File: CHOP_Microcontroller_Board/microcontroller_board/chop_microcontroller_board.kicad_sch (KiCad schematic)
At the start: 33 parts, among them J11 HEATER_SIGNAL_1, J12 POWER_HEAT, J14 BatteryToMainBoard, J2 OLED, J3 Encoder, J6 PFLOW, J7 DISC PUMP, J8 RTC, U1 Teensy4.1_Mounted, U2 U3V50F24, U3 U3V50F12, U4 D36V6F5

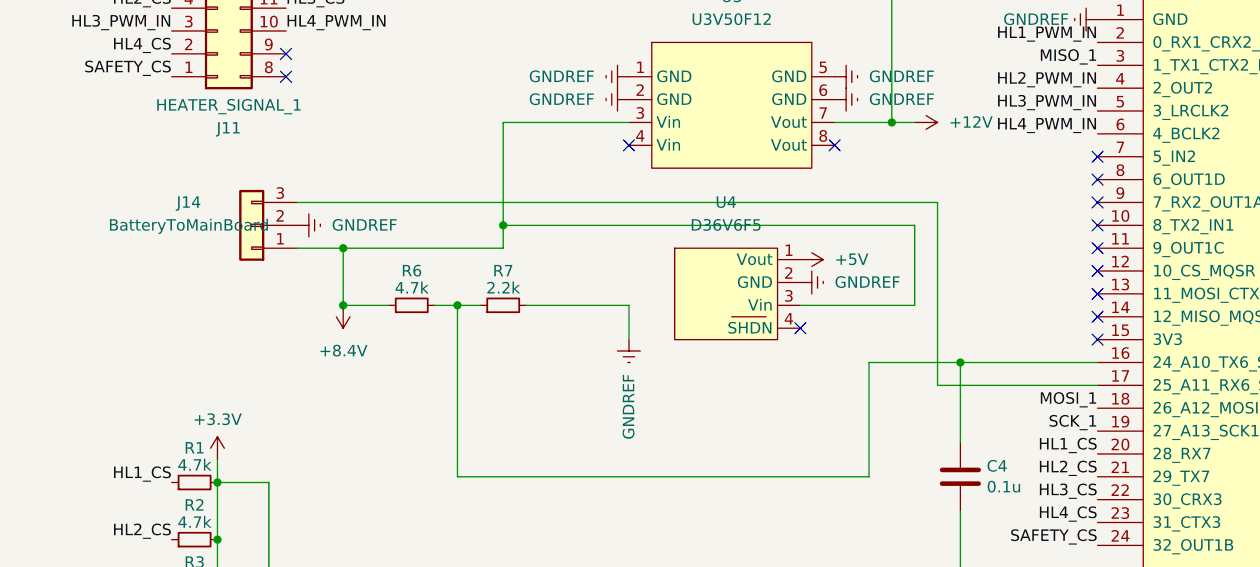
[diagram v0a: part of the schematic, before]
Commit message: CHOP 3d models 5/30
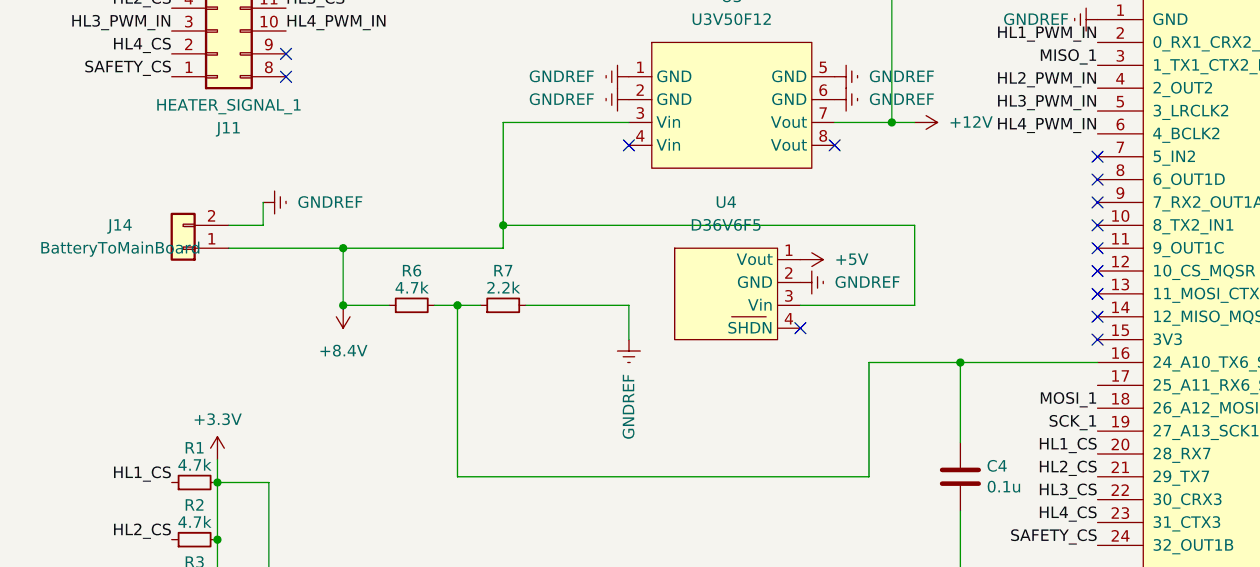
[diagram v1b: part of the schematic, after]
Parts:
- J14: footprint Connector_JST:JST_PH_S3B-PH-K_1x03_P2.00mm_Horizontal -> Connector_JST:JST_PH_S2B-PH-K_1x02_P2.00mm_Horizontal; symbol Connector_Generic:Conn_01x03 -> Connector_Generic:Conn_01x02
- J2: footprint Connector_PinHeader_2.54mm:PinHeader_1x04_P2.54mm_Vertical -> chop_footprint_library:128x64OLED
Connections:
- net at U1.17 (25_A11_RX6_SDA2): no longer J14.3 (Pin_3)
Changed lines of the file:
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@@
 	(wire
 		(pts
-			(xy 43.18 77.47) (xy 48.26 77.47)
-		)
-		(stroke
-			(width 0)
-			(type default)
-		)
-	)
-	(wire
-		(pts
 			(xy 40.005 103.505) (xy 40.005 147.955)
 		)
@@
 	(wire
 		(pts
-			(xy 114.3 72.39) (xy 114.3 92.71)
-		)
-		(stroke
-			(width 0)
-			(type default)
-		)
-	)
-	(wire
-		(pts
 			(xy 16.51 27.305) (xy 23.495 27.305)
 		)
@@
 	(wire
 		(pts
-			(xy 114.3 92.71) (xy 132.08 92.71)
-		)
-		(stroke
-			(width 0)
-			(type default)
-		)
-	)
-	(wire
-		(pts
 			(xy 38.735 29.845) (xy 36.195 29.845)
 		)
@@
 	(wire
 		(pts
+			(xy 35.56 77.47) (xy 48.26 77.47)
+		)
+		(stroke
+			(width 0)
+			(type default)
+		)
+	)
+	(wire
+		(pts
 			(xy 99.06 83.82) (xy 111.76 83.82)
 		)
@@
 	(wire
 		(pts
+			(xy 39.37 74.93) (xy 39.37 72.39)
+		)
+		(stroke
+			(width 0)
+			(type default)
+		)
+	)
+	(wire
+		(pts
 			(xy 34.29 100.965) (xy 34.29 103.505)
 		)
@@
 	(wire
 		(pts
-			(xy 43.18 72.39) (xy 114.3 72.39)
+			(xy 144.78 152.4) (xy 144.78 147.32)
 		)
 		(stroke
@@
 	(wire
 		(pts
-			(xy 144.78 152.4) (xy 144.78 147.32)
+			(xy 35.56 74.93) (xy 39.37 74.93)
 		)
 		(stroke
@@
 			)
 		)
-		(property "Footprint" "Connector_PinHeader_2.54mm:PinHeader_1x04_P2.54mm_Vertical"
+		(property "Footprint" "chop_footprint_library:128x64OLED"
 			(at 170.18 147.32 0)
 			(effects
@@
 	(symbol
 		(lib_id "power:GNDREF")
-		(at 43.18 74.93 90)
+		(at 39.37 72.39 90)
 		(unit 1)
 		(exclude_from_sim no)
@@
 		(dnp no)
 		(property "Reference" "#PWR091"
-			(at 49.53 74.93 0)
+			(at 45.72 72.39 0)
 			(effects
 				(font
@@
 		)
 		(property "Value" "GNDREF"
-			(at 46.99 74.93 90)
+			(at 43.18 72.39 90)
 			(effects
 				(font
@@
 		)
 		(property "Footprint" ""
-			(at 43.18 74.93 0)
+			(at 39.37 72.39 0)
 			(effects
 				(font
@@
 		)
 		(property "Datasheet" ""
-			(at 43.18 74.93 0)
+			(at 39.37 72.39 0)
 			(effects
 				(font
@@
 		)
 		(property "Description" ""
-			(at 43.18 74.93 0)
+			(at 39.37 72.39 0)
 			(effects
 				(font
@@
 	)
 	(symbol
-		(lib_id "Connector_Generic:Conn_01x03")
-		(at 38.1 74.93 180)
+		(lib_id "Connector_Generic:Conn_01x02")
+		(at 30.48 77.47 180)
 		(unit 1)
 		(exclude_from_sim no)
@@
 		(dnp no)
 		(property "Reference" "J14"
-			(at 31.115 72.39 0)
+			(at 23.495 74.93 0)
 			(effects
 				(font
@@
 		)
 		(property "Value" "BatteryToMainBoard"
-			(at 31.115 74.93 0)
+			(at 23.495 77.47 0)
 			(effects
 				(font
@@
 			)
 		)
-		(property "Footprint" "Connector_JST:JST_PH_S3B-PH-K_1x03_P2.00mm_Horizontal"
-			(at 38.1 74.93 0)
+		(property "Footprint" "Connector_JST:JST_PH_S2B-PH-K_1x02_P2.00mm_Horizontal"
+			(at 30.48 77.47 0)
 			(effects
 				(font
@@
 		)
 		(property "Datasheet" "~"
-			(at 38.1 74.93 0)
+			(at 30.48 77.47 0)
 			(effects
 				(font
@@
 			)
 		)
-		(property "Description" "Generic connector, single row, 01x03, script generated (kicad-library-utils/schlib/autogen/connector/)"
-			(at 38.1 74.93 0)
+		(property "Description" "Generic connector, single row, 01x02, script generated (kicad-library-utils/schlib/autogen/connector/)"
+			(at 30.48 77.47 0)
 			(effects
 				(font
@@
 		(pin "2"
 		)
-		(pin "3"
-		)
 		(instances
